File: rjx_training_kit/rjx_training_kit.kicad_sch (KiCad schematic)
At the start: 21 parts, among them J1 Barrel_Jack_Switch, J2 Conn_02x03, J3 ST-Link, SW1 SW_SPDT, U1 TLV76133DCY, U2 LM2596S-ADJ

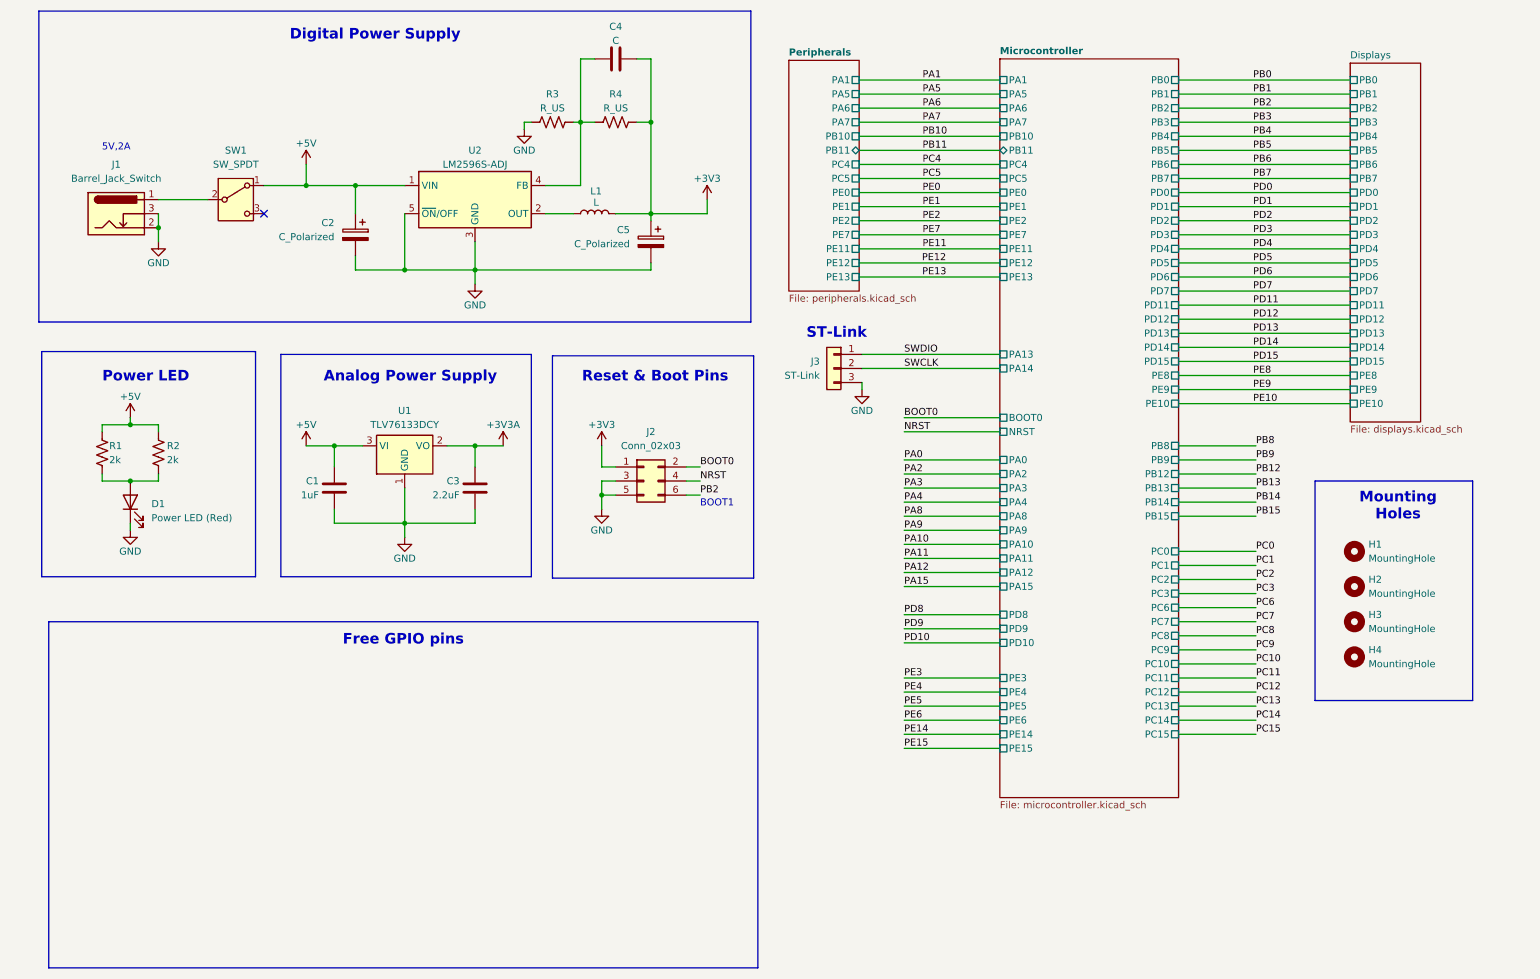
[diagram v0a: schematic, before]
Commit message: Update
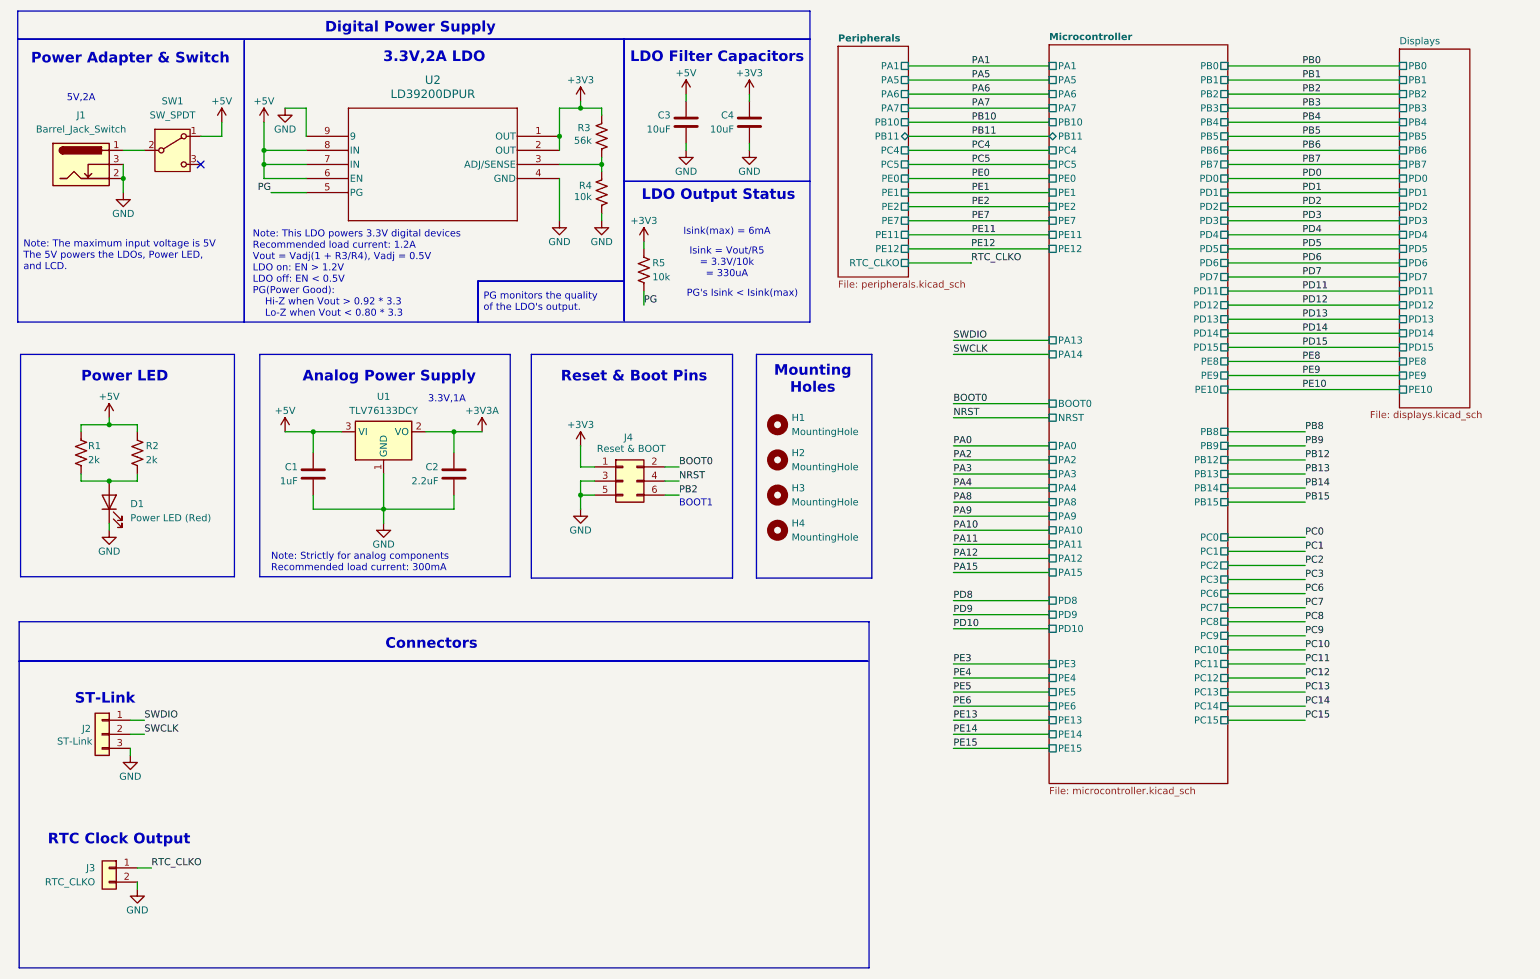
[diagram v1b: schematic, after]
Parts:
- removed C2, C5: C_Polarized, symbol Device:C_Polarized
- removed J3: ST-Link, symbol Connector_Generic:Conn_01x03
- removed L1: L, symbol Device:L
- removed U2: LM2596S-ADJ, Package_TO_SOT_SMD:TO-263-5_TabPin3, symbol Regulator_Switching:LM2596S-ADJ
- added C3: 10uF, symbol Device:C
- added J2: ST-Link, symbol Connector_Generic:Conn_01x03
- added J3: RTC_CLKO, symbol Connector_Generic:Conn_01x02
- added R5: 10k, symbol Device:R_US
- added U2: LD39200DPUR, LD39200:DFN-8-1EP_4x4mm_P0.8mm_EP2.3x3.24mm, symbol Regulator_LDO:LD39200DPUR
- C4: value C -> 10uF
- J4: renamed from J2; value Conn_02x03 -> Reset & BOOT
- R3: value R_US -> 56k
- R4: value R_US -> 10k
- renumbered C3 to C2
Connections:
- net +3V3: now also C4.1, R3.2, R5.1, U2.1 (OUT), U2.2 (OUT); no longer C4.2, R4.2
- net +5V: now also C3.1, U2.6 (EN), U2.7 (IN), U2.8 (IN)
- net GND: now also C4.2, R4.1, C3.2, J2.3 (Pin_3), J3.2 (Pin_2), U2.4 (GND), U2.9; no longer R3.1
- net SWCLK: now also J2.2 (Pin_2)
- net SWDIO: now also J2.1 (Pin_1)
- new net: R3.1, R4.2, U2.3 (ADJ/SENSE)
- new net PG: R5.2, U2.5 (PG)
- new net RTC_CLKO: J3.1 (Pin_1)
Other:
- sheet Peripherals ports: added RTC_CLKO; removed PE13
- note added: "3.3V,1A"
- note added: "3.3V,2A LDO"
- note added: "Connectors"
- note added: "Isink = Vout/R5 = 3.3V/10k = 330uA"
- note added: "Isink(max) = 6mA"
- note added: "LDO Filter Capacitors"
- note added: "LDO Output Status"
- note added: "Note: Strictly for analog components Recommended load current: 300mA"
- note added: "Note: The maximum input voltage is 5V The 5V powers the LDOs, Power LED, and LCD."
- note added: "Note: This LDO powers 3.3V digital devices Recommended load current: 1.2A Vout = Vadj(1 + R3/R4), Vadj = 0.5V LDO on: EN > 1.2V LDO off: EN < 0.5V PG(Power Good): Hi-Z when Vout > 0.92 * 3.3 Lo-Z when Vout < 0.80 * 3.3"
- note added: "PG monitors the quality of the LDO's output."
- note added: "PG's Isink < Isink(max)"
- note added: "Power Adapter & Switch"
- note added: "RTC Clock Output"
- note removed: "Free GPIO pins"
- moved on the sheet: C1, C2, D1, J1, J4, R1, R2, SW1, U1
